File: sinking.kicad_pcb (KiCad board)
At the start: 2 copper layers, 142.2 x 86.4 mm, 14 parts, among them Q1 Q_NPN_BCE, U1 LTV-817, U2 V7805-1000, U3 INA219AxD, U4 74HC14

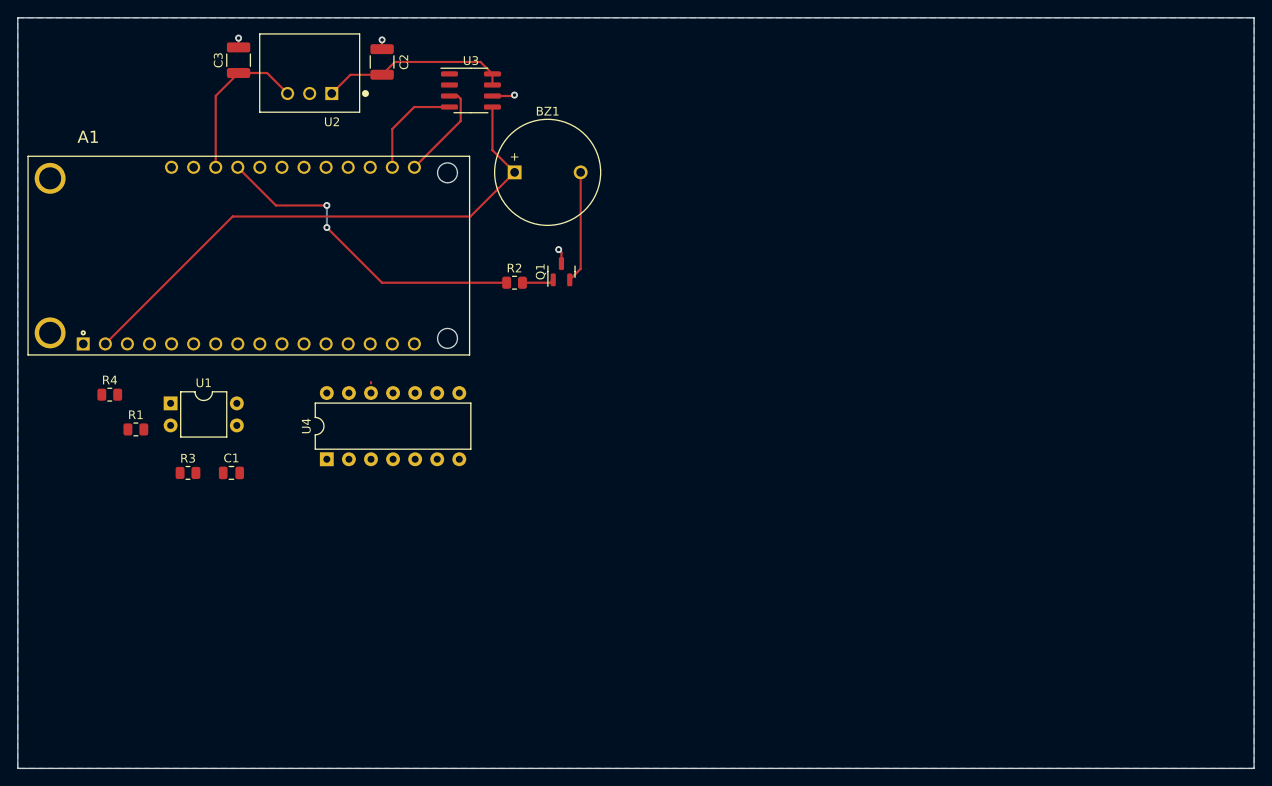
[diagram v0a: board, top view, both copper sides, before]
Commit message: first layout
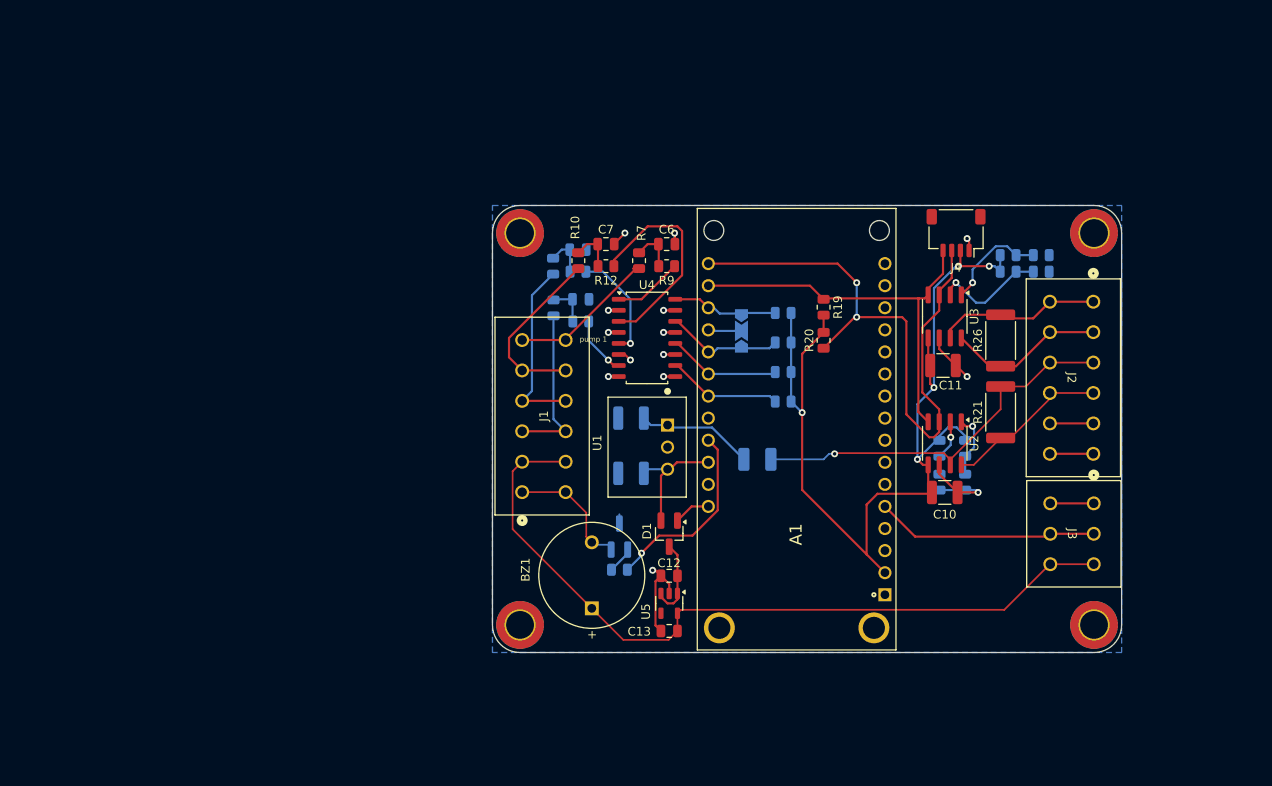
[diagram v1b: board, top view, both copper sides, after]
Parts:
- removed C3: 22u, Capacitor_SMD:C_1210_3225Metric
- removed R2: 1k, Resistor_SMD:R_0805_2012Metric
- removed R3: 10k, Resistor_SMD:R_0805_2012Metric
- removed R4: 5k, Resistor_SMD:R_0805_2012Metric
- added C10: 0.1u, Capacitor_SMD:C_1210_3225Metric, F.Cu at (165.1, 95.2)
- added C11: 0.1u, Capacitor_SMD:C_1210_3225Metric, F.Cu at (164.9, 80.6)
- added C12: 1u, Capacitor_SMD:C_0805_2012Metric, F.Cu at (133.4, 104.8)
- added C13: 1u, Capacitor_SMD:C_0805_2012Metric, F.Cu at (133.4, 111.2)
- added C6: 4.7u, Capacitor_SMD:C_0805_2012Metric, F.Cu at (133.1, 66.7)
- added C7: 4.7u, Capacitor_SMD:C_0805_2012Metric, F.Cu at (126.1, 66.7)
- added C8: 4.7u, Capacitor_SMD:C_0805_2012Metric, B.Cu at (122.9, 67.3)
- added C9: 4.7u, Capacitor_SMD:C_0805_2012Metric, B.Cu at (123.2, 73.0)
- added D1: PMEG2005, Package_TO_SOT_SMD:SOT-23_Handsoldering, F.Cu at (133.4, 100.0)
- added J1: 1861975, 1891975:CONN_1861975, F.Cu at (121.4, 77.7)
- added J2: 1861975, 1891975:CONN_1861975, F.Cu at (177.2, 90.8)
- added J3: 1861946, 1891946:CONN_1861946, F.Cu at (177.2, 103.5)
- added J4: SM04B-SRSS-TB, Connector_JST:JST_SH_SM04B-SRSS-TB_1x04-1MP_P1.00mm_Horizontal, F.Cu at (166.4, 65.4)
- added JP1: SolderJumper_3_Open, Jumper:SolderJumper-3_P2.0mm_Open_TrianglePad1.0x1.5mm, B.Cu at (141.7, 76.7)
- added R10: 2.2k, Resistor_SMD:R_0805_2012Metric, F.Cu at (122.9, 68.6)
- added R11: 4.7k, Resistor_SMD:R_0805_2012Metric, B.Cu at (146.5, 78.0)
- added R12: 2.2k, Resistor_SMD:R_0805_2012Metric, F.Cu at (126.1, 69.2)
- added R13: 2.2k, Resistor_SMD:R_0805_2012Metric, B.Cu at (120.0, 69.2)
- added R14: 4.7k, Resistor_SMD:R_0805_2012Metric, B.Cu at (146.5, 81.4)
- added R15: 2.2k, Resistor_SMD:R_0805_2012Metric, B.Cu at (122.9, 69.8)
- added R16: 2.2k, Resistor_SMD:R_0805_2012Metric, B.Cu at (120.1, 74.0)
- added R17: 4.7k, Resistor_SMD:R_0805_2012Metric, B.Cu at (146.5, 84.8)
- added R18: 2.2k, Resistor_SMD:R_0805_2012Metric, B.Cu at (123.2, 75.6)
- added R19: 10k, Resistor_SMD:R_0805_2012Metric, F.Cu at (151.1, 73.9)
- added R20: 10k, Resistor_SMD:R_0805_2012Metric, F.Cu at (151.1, 77.7)
- added R21: 0.1, Resistor_SMD:R_2512_6332Metric, F.Cu at (171.5, 86.0)
- added R22: 10k, Resistor_SMD:R_0805_2012Metric, B.Cu at (167.4, 94.1)
- added R23: 10k, Resistor_SMD:R_0805_2012Metric, B.Cu at (164.5, 94.1)
- added R24: 0, Resistor_SMD:R_1210_3225Metric_Pad1.30x2.65mm_HandSolder, B.Cu at (143.5, 91.4)
- added R25: 10k, Resistor_SMD:R_0805_2012Metric, B.Cu at (167.4, 90.2)
- added R26: 0.1, Resistor_SMD:R_2512_6332Metric, F.Cu at (171.5, 77.8)
- added R27: 10k, Resistor_SMD:R_0805_2012Metric, B.Cu at (176.2, 67.9)
- added R28: 10k, Resistor_SMD:R_0805_2012Metric, B.Cu at (176.2, 69.8)
- added R29: 10k, Resistor_SMD:R_0805_2012Metric, B.Cu at (164.5, 90.2)
- added R30: 10k, Resistor_SMD:R_0805_2012Metric, B.Cu at (172.4, 67.9)
- added R31: 10k, Resistor_SMD:R_0805_2012Metric, B.Cu at (172.4, 69.8)
- added R7: 2.2k, Resistor_SMD:R_0805_2012Metric, F.Cu at (129.9, 68.6)
- added R8: 4.7k, Resistor_SMD:R_0805_2012Metric, B.Cu at (146.5, 74.6)
- added R9: 2.2k, Resistor_SMD:R_0805_2012Metric, F.Cu at (133.1, 69.2)
- added REF**: MountingHole_3.2mm_M3_ISO14580_Pad_TopBottom, MountingHole:MountingHole_3.2mm_M3_ISO14580_Pad_TopBottom, F.Cu at (182.2, 65.4)
- added REF**: MountingHole_3.2mm_M3_ISO14580_Pad_TopBottom, MountingHole:MountingHole_3.2mm_M3_ISO14580_Pad_TopBottom, F.Cu at (116.2, 65.4)
- added REF**: MountingHole_3.2mm_M3_ISO14580_Pad_TopBottom, MountingHole:MountingHole_3.2mm_M3_ISO14580_Pad_TopBottom, F.Cu at (182.2, 110.5)
- added REF**: MountingHole_3.2mm_M3_ISO14580_Pad_TopBottom, MountingHole:MountingHole_3.2mm_M3_ISO14580_Pad_TopBottom, F.Cu at (116.2, 110.5)
- added U5: TPS7A2033PDBVR, Package_TO_SOT_SMD:SOT-23-5, F.Cu at (133.4, 108.0)
- A1: footprint boron:Boron -> libs:Boron
- C1: value 1u -> 10u; footprint Capacitor_SMD:C_0805_2012Metric -> Capacitor_SMD:C_1210_3225Metric; moved to B.Cu
- C2: value 10u -> 22u; moved to B.Cu
- Q1: footprint Package_TO_SOT_SMD:SOT-23 -> Package_TO_SOT_SMD:SOT-23_Handsoldering; moved to B.Cu
- R1: value 5k -> 1k; moved to B.Cu
- U1: value LTV-817 -> V7805-1000; footprint Package_DIP:DIP-4_W7.62mm -> libs:CONV_V7805-1000
- U2: value V7805-1000 -> INA219AxD; footprint libs:CONV_V7805-1000 -> Package_SO:SOIC-8_3.9x4.9mm_P1.27mm
- U4: value 74HC14 -> TLP291-4; footprint Package_DIP:DIP-14_W7.62mm -> Package_SO:SOIC-16_4.55x10.3mm_P1.27mm
- moved U2 84.6 mm to (165.1, 89.6), turned to -90 degrees
- moved A1 66.1 mm to (148.0, 88.0), turned to 90 degrees
- moved U3 60.4 mm to (165.1, 75.0), turned to -90 degrees
- moved R1 57.9 mm to (127.6, 104.1), turned to 180 degrees
- moved C2 55.3 mm to (129.0, 93.0), turned to 180 degrees
- moved U1 55.1 mm to (130.8, 90.0), turned to -90 degrees
- moved BZ1 50.9 mm to (124.5, 108.6), turned to 90 degrees
- moved C1 46.4 mm to (129.0, 86.7), turned to 180 degrees
- moved U4 39.4 mm to (130.8, 77.5), turned to 0 degrees
- moved Q1 31.2 mm to (127.6, 100.3)
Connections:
- net Net-(BZ1--) renamed buzzer -
- A1 pad A0: unconnected-(A1-19_P0.03_PWM2_ADC0-PadA0) -> water_sense_sig
- A1 pad D2: Net-(A1-SDA1_UART1_RTS_SPI1_SCK_PWM3_P1.01_2) -> /input_filter/out
- A1 pad D3: unconnected-(A1-SCL1_UART1_CTS_SPI1_MOSI_PWM3_P1.02_3-PadD3) -> Net-(A1-SCL1_UART1_CTS_SPI1_MOSI_PWM3_P1.02_3)
- A1 pad D4: unconnected-(A1-UART2_TX_SPI1_MISO_PWM1_P1.08_4-PadD4) -> /input_filter1/out
- A1 pad D5: unconnected-(A1-UART2_RX_PWM1_P1.10_5-PadD5) -> /input_filter2/out
- A1 pad D6: unconnected-(A1-UART2_CTS_PWM1_P1.11_6-PadD6) -> /input_filter3/out
- A1 pad LI+: unconnected-(A1-LiPo+-PadLI+) -> Net-(A1-LiPo+)
- A1 pad SCL: Net-(A1-1_SCL_P0.27) -> SCL
- A1 pad SDA: Net-(A1-0_SDA_P0.26) -> SDA
- A1 pad VUSB: VUSB -> /VUSB
- BZ1 pad 1: +3V3 -> buzzer +
- C1 pad 1: Net-(C1-Pad1) -> Net-(U1-+VIN)
- C2 pad 1: +12V -> /VUSB
- R1 pad 1: Net-(R1-Pad1) -> Net-(A1-UART2_RTS_PWM1_P1.03_8)
- R1 pad 2: bilge_pump_pos -> Net-(Q1-B)
- U1 pad 1: Net-(R1-Pad1) -> Net-(U1-+VIN)
- U1 pad 3: GND -> /VUSB
- U2 pad 1: +12V -> Net-(U2-A1)
- U2 pad 2: GND -> Net-(U2-A0)
- U2 pad 3: VUSB -> SDA
- U3 pad 1: unconnected-(U3-A1-Pad1) -> Net-(U3-A1)
- U3 pad 2: unconnected-(U3-A0-Pad2) -> Net-(U3-A0)
- U3 pad 3: Net-(A1-0_SDA_P0.26) -> SDA
- U3 pad 4: Net-(A1-1_SCL_P0.27) -> SCL
- U3 pad 7: +12V -> aux_bat_sense_-
- U3 pad 8: +12V -> aux_bat_sese_+
- U4 pad 1: (no net) -> Net-(R9-Pad1)
- U4 pad 10: (no net) -> /input_filter3/out
- U4 pad 11: (no net) -> GND
- U4 pad 12: Net-(A1-SDA1_UART1_RTS_SPI1_SCK_PWM3_P1.01_2) -> /input_filter2/out
- U4 pad 13: Net-(C1-Pad1) -> GND
- U4 pad 14: +3V3 -> /input_filter1/out
- U4 pad 2: (no net) -> GND
- U4 pad 3: (no net) -> Net-(R12-Pad1)
- U4 pad 4: (no net) -> GND
- U4 pad 5: (no net) -> Net-(R15-Pad1)
- U4 pad 6: (no net) -> GND
- U4 pad 7: GND -> Net-(R18-Pad1)
- U4 pad 8: (no net) -> GND
- U4 pad 9: (no net) -> GND
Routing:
- net buzzer +: track 0.00 -> 90.6 mm
- net SDA: track 0.00 -> 72.1 mm, vias 0 -> 2
- net +3V3: track 63.8 -> 112.7 mm, vias 0 -> 5
- net SCL: track 0.00 -> 46.7 mm
- net +12V_IN_-: track 0.00 -> 44.5 mm, vias 0 -> 1
- net GND: track 6.45 -> 49.6 mm, vias 4 -> 14
- net water_sense_sig: track 0.00 -> 25.6 mm
- net Net-(R12-Pad1): track 0.00 -> 25.0 mm
- net +12V: track 22.2 -> 0.00 mm
- net engine_running: track 0.00 -> 21.1 mm
- net bilge_pump_2_running: track 0.00 -> 20.7 mm
- net aux_bat_sense_-: track 0.00 -> 19.1 mm
- net +12V_IN_+: track 0.00 -> 19.0 mm
- net aux_input: track 0.00 -> 18.9 mm
- net VUSB: track 18.6 -> 0.00 mm
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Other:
- board size 142.2 x 86.4 mm -> 72.4 x 51.4 mm
- board text added: "pump 1"
